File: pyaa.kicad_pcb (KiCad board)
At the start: 2 copper layers, 123 x 80.1 mm, 18 parts, among them J1 MJ-4PP-9, K0 KEYSW, K1 KEYSW, SW1 SW_PUSH, U1 ProMicro

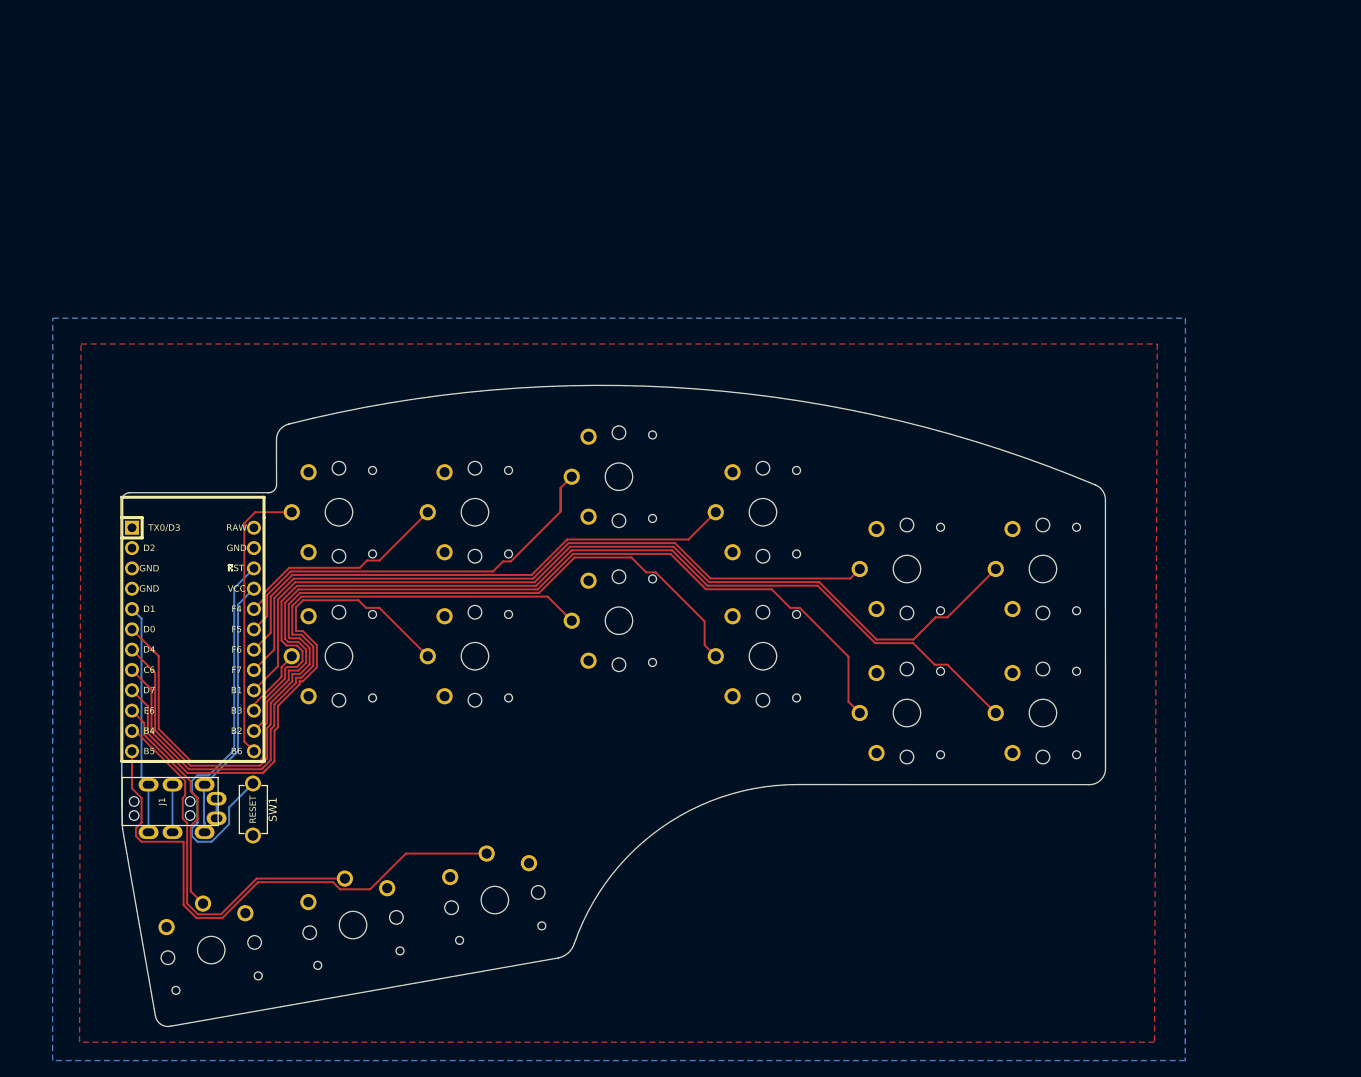
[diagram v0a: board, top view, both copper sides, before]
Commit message: Add files via upload
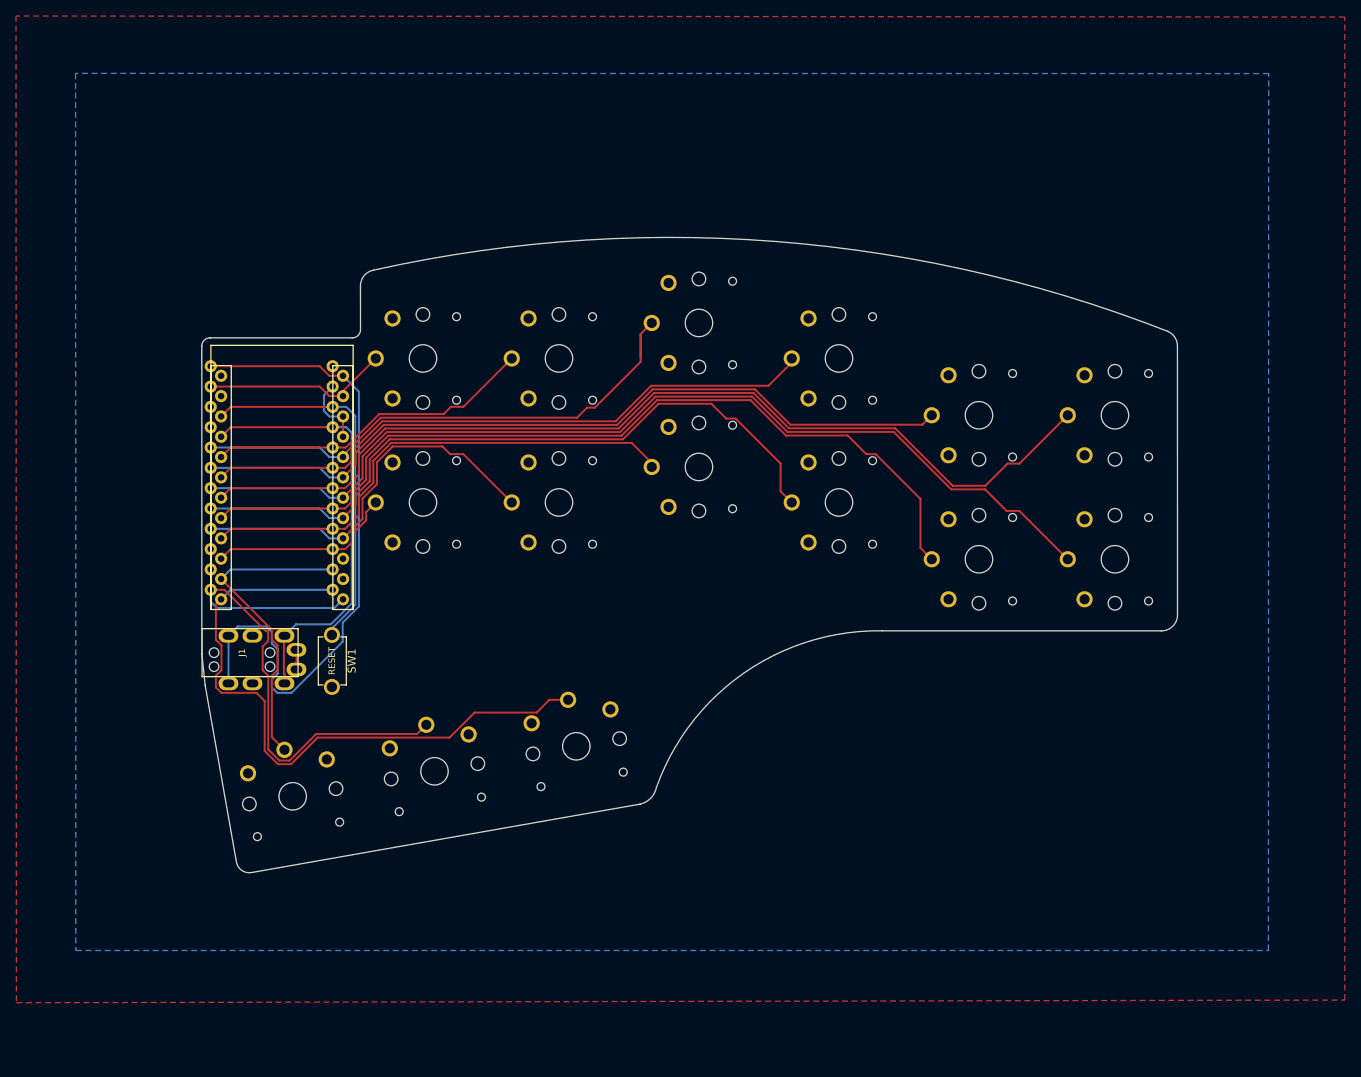
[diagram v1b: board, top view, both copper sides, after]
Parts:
- U1: footprint Keebio-Parts:ArduinoProMicro -> Lily58-footprint:ProMicro_rev2
- moved U1 22.3 mm to (101.5, 91.0), turned to 0 degrees
- moved KHL1 21.9 mm to (136.2, 75.2)
- moved KRL1 21.9 mm to (136.2, 93.2)
- moved KST1 21.9 mm to (119.2, 75.2)
- moved KST2 21.9 mm to (119.2, 93.2)
- moved KN1 21.7 mm to (138.4, 123.7)
- moved KA1 21.7 mm to (120.7, 126.8)
- moved KO1 21.7 mm to (103.0, 129.9)
- moved KPL1 21.7 mm to (153.8, 70.8)
- moved KWL1 21.7 mm to (153.8, 88.8)
- moved KKL1 21.4 mm to (171.2, 93.2)
- moved KTL1 21.4 mm to (171.2, 75.2)
- moved K0 21.2 mm to (205.8, 82.3)
- moved K1 21.2 mm to (205.8, 100.3)
- moved KS1 21.2 mm to (188.8, 82.3)
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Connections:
- U1 pad 1: Net-(U1-Pad1) -> Net-(J1-PadB)
- U1 pad 10: Net-(KO1-Pad1) -> Net-(U1-Pad10)
- U1 pad 11: Net-(KA1-Pad1) -> Net-(U1-Pad11)
- U1 pad 12: Net-(KN1-Pad1) -> Net-(KA1-Pad1)
- U1 pad 13: Net-(KST1-Pad1) -> Net-(KN1-Pad1)
- U1 pad 14: Net-(K1-Pad1) -> Net-(KO1-Pad1)
- U1 pad 16: Net-(K0-Pad1) -> Net-(KWL1-Pad1)
- U1 pad 17: Net-(KS1-Pad1) -> Net-(KS2-Pad1)
- U1 pad 18: Net-(KTL1-Pad1) -> Net-(K0-Pad1)
- U1 pad 19: Net-(KPL1-Pad1) -> Net-(KTL1-Pad1)
- U1 pad 2: Net-(U1-Pad2) -> Net-(KST1-Pad1)
- U1 pad 5: Net-(J1-PadB) -> Net-(KPL1-Pad1)
- U1 pad 6: Net-(KS2-Pad1) -> Net-(KS1-Pad1)
- U1 pad 7: Net-(KKL1-Pad1) -> Net-(K1-Pad1)
- U1 pad 8: Net-(KWL1-Pad1) -> Net-(KKL1-Pad1)
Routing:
- net Net-(J1-PadB): track 28.8 -> 83.4 mm
- net Net-(KS2-Pad1): track 138.8 -> 108.9 mm
- net Net-(KKL1-Pad1): track 114.0 -> 88.5 mm
- net Net-(KWL1-Pad1): track 86.5 -> 63.4 mm
- net VDD: track 33.1 -> 54.6 mm
- net Net-(KRL1-Pad1): track 68.0 -> 48.9 mm
- net Net-(KA1-Pad1): track 47.4 -> 65.7 mm
- net Net-(KST2-Pad1): track 8.76 -> 23.4 mm
- net Net-(KHL1-Pad1): track 27.2 -> 41.4 mm
- net Net-(KPL1-Pad1): track 53.9 -> 67.7 mm
- net Net-(KN1-Pad1): track 68.1 -> 81.3 mm
- net Net-(KST1-Pad1): track 35.5 -> 23.4 mm
- net Net-(KTL1-Pad1): track 67.5 -> 78.7 mm
- net Net-(KO1-Pad1): track 28.5 -> 39.7 mm
- net Net-(KS1-Pad1): track 88.4 -> 98.4 mm
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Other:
- board size 123 x 80.1 mm -> 122 x 79.4 mm
